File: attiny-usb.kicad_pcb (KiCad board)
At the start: 2 copper layers, 40 x 12.2 mm, 12 parts, among them J1 Conn_01x05, U1 ATtiny85-20P

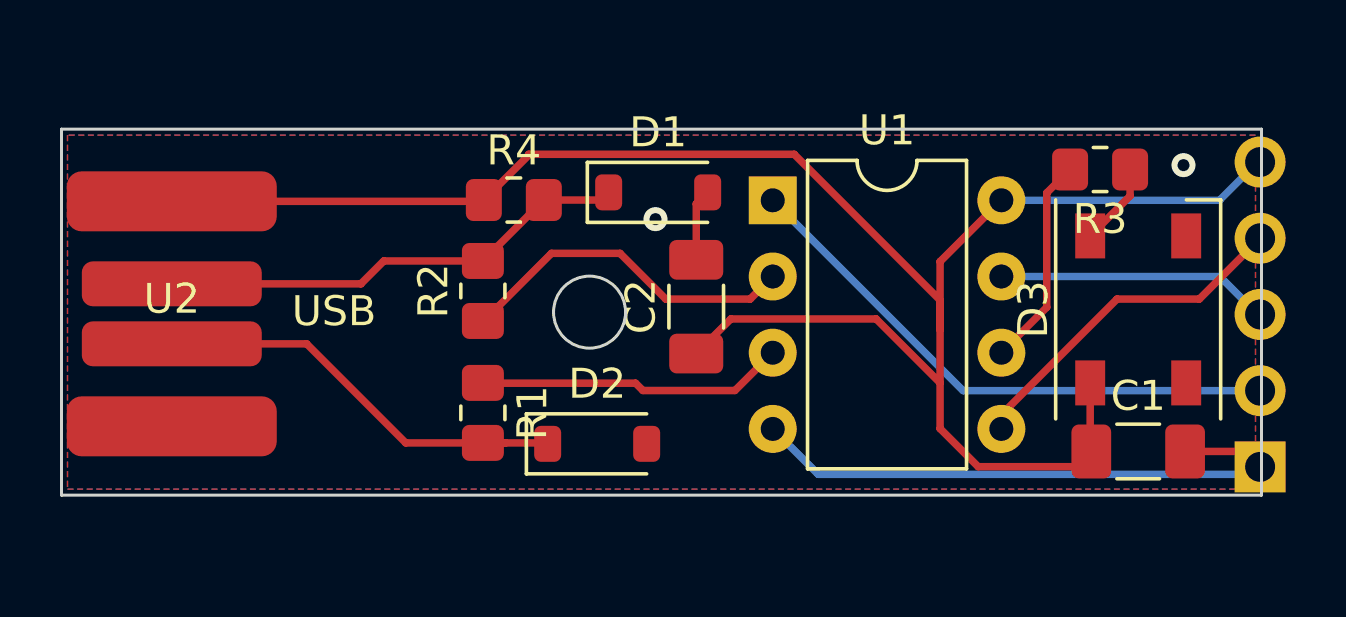
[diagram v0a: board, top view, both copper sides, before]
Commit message: design new pcb
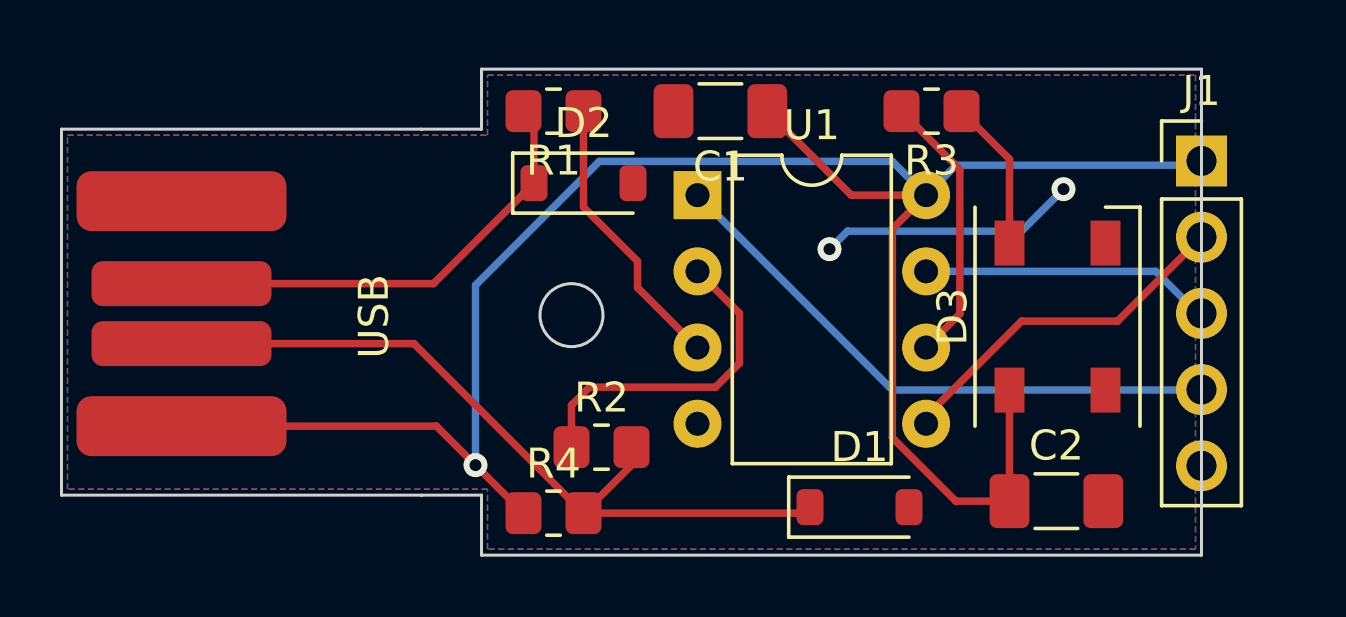
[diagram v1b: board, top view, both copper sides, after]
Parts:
- moved C1 18.0 mm to (122.0, 99.4), turned to 180 degrees
- moved C2 13.6 mm to (133.2, 112.4), turned to 0 degrees
- moved D1 12.5 mm to (126.6, 112.6)
- moved R4 10.5 mm to (116.4, 112.8)
- moved R1 10.3 mm to (116.4, 99.4), turned to 180 degrees
- moved D2 8.70 mm to (117.4, 101.8)
- moved R2 6.54 mm to (118.0, 110.6), turned to 0 degrees
- moved R3 5.95 mm to (129.0, 99.4)
- moved D3 2.70 mm to (133.2, 106.2)
- moved U1 2.51 mm to (121.2, 102.2)
- moved J1 1.95 mm to (138.0, 101.1)
- moved U2 0.32 mm to (104.0, 106.2)
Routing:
- net GND: track 22.0 -> 8.63 mm
- net Net-(D1-K): track 15.8 -> 26.2 mm
- net +5V: track 64.4 -> 68.9 mm, vias 0 -> 1
- net Net-(D3-DIN): track 2.76 -> 5.06 mm
- net Net-(U1-PB1): track 7.06 -> 9.15 mm
- net Net-(D2-K): track 14.7 -> 15.7 mm
- net Net-(U1-XTAL2/PB4): track 10.3 -> 9.45 mm
- net Net-(J1-Pin_3): track 9.07 -> 9.63 mm
- net Net-(J1-Pin_4): track 18.9 -> 19.4 mm
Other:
- board size 40 x 12.2 mm -> 38 x 16.2 mm
